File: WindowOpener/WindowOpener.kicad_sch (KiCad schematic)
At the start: 32 parts, among them J1 Conn_ST_STDC14, J2 UEXT_Host, SW1 SW_Push, SW2 SW_SPDT_XKB, U1 STM32L152RCTxA, Y1 8MHz, Y2 32.768kHz

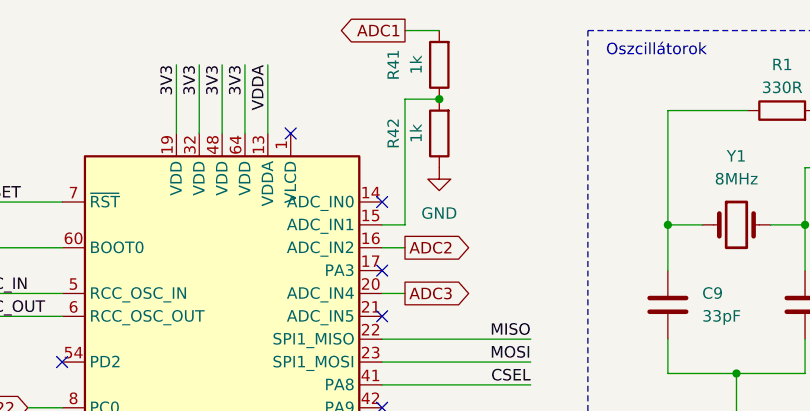
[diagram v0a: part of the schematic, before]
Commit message: v0.5
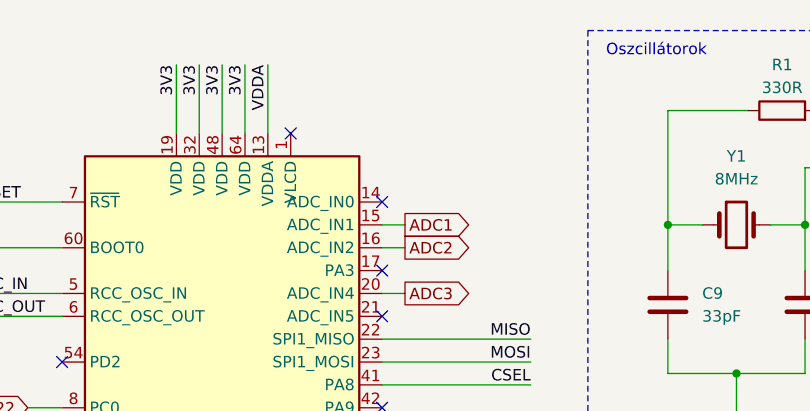
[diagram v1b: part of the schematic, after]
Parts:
- removed R41, R42: 1k, Resistor_SMD:R_2010_5025Metric_Pad1.40x2.65mm_HandSolder, symbol Device:R
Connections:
- net ADC1: now also U1.15 (PA1)

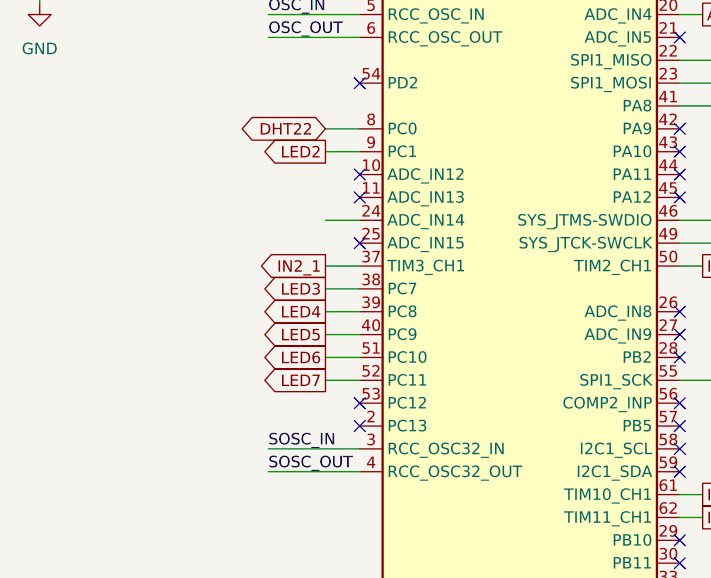
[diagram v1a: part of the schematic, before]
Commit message: v0.6
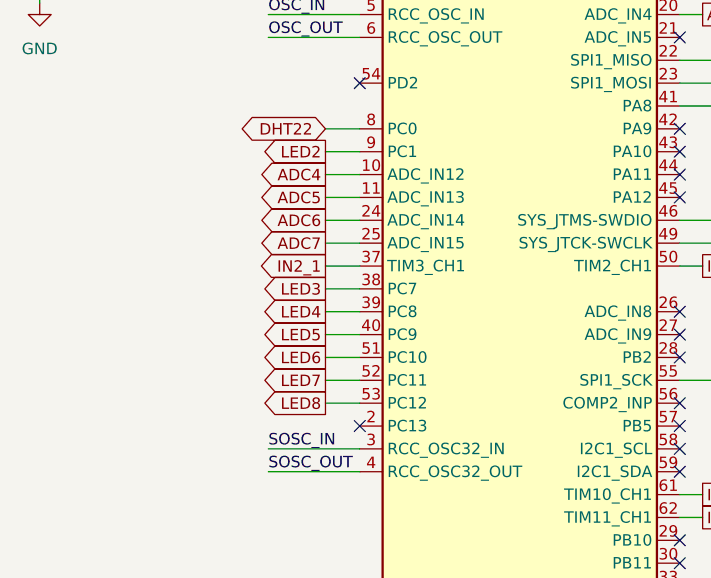
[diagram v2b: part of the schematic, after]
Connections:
- net ADC4: now reaches U1.10 (PC2)
- net ADC5: now reaches U1.11 (PC3)
- net ADC6: now reaches U1.24 (PC4)
- net ADC7: now reaches U1.25 (PC5)
- net LED8: now reaches U1.53 (PC12)
- no-connect marks 27 -> 23
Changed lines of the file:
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@@
-	)
-	(no_connect
-		(at 76.2 86.36)
 	)
 	(no_connect
@@
 	)
 	(no_connect
-		(at 76.2 60.96)
-	)
-	(no_connect
 		(at 111.76 86.36)
 	)
@@
 	)
 	(no_connect
-		(at 76.2 68.58)
-	)
-	(no_connect
 		(at 111.76 55.88)
 	)
@@
 		(at 111.76 63.5)
 	)
-	(no_connect
-		(at 76.2 63.5)
-	)
 	(wire
 		(pts
@@
 	(wire
 		(pts
+			(xy 72.39 60.96) (xy 76.2 60.96)
+		)
+		(stroke
+			(width 0)
+			(type default)
+		)
+	)
+	(wire
+		(pts
 			(xy 96.52 17.78) (xy 96.52 25.4)
 		)
@@
 	(wire
 		(pts
+			(xy 72.39 66.04) (xy 76.2 66.04)
+		)
+		(stroke
+			(width 0)
+			(type default)
+		)
+	)
+	(wire
+		(pts
 			(xy 182.88 107.95) (xy 185.42 107.95)
 		)
@@
 	(wire
 		(pts
+			(xy 72.39 68.58) (xy 76.2 68.58)
+		)
+		(stroke
+			(width 0)
+			(type default)
+		)
+	)
+	(wire
+		(pts
 			(xy 271.78 120.65) (xy 280.67 120.65)
 		)
@@
 	(wire
 		(pts
+			(xy 72.39 63.5) (xy 76.2 63.5)
+		)
+		(stroke
+			(width 0)
+			(type default)
+		)
+	)
+	(wire
+		(pts
 			(xy 72.39 58.42) (xy 76.2 58.42)
 		)
@@
 	(wire
 		(pts
+			(xy 72.39 86.36) (xy 76.2 86.36)
+		)
+		(stroke
+			(width 0)
+			(type default)
+		)
+	)
+	(wire
+		(pts
 			(xy 165.1 118.11) (xy 167.64 118.11)
 		)
@@
 		(pts
 			(xy 250.19 44.45) (xy 250.19 49.53)
-		)
-		(stroke
-			(width 0)
-			(type default)
-		)
-	)
-	(wire
-		(pts
-			(xy 72.39 66.04) (xy 76.2 66.04)
 		)
 		(stroke
@@
 			)
 			(justify left bottom)
+		)
+	)
+	(global_label "LED8"
+		(shape output)
+		(at 72.39 86.36 180)
+		(fields_autoplaced yes)
+		(effects
+			(font
+				(size 1.27 1.27)
+			)
+			(justify right)
+		)
+		(property "Intersheetrefs" "${INTERSHEET_REFS}"
+			(at 64.7482 86.36 0)
+			(effects
+				(font
+					(size 1.27 1.27)
+				)
+				(justify right)
+				(hide yes)
+			)
+		)
+	)
+	(global_label "ADC5"
+		(shape output)
+		(at 72.39 63.5 180)
+		(fields_autoplaced yes)
+		(effects
+			(font
+				(size 1.27 1.27)
+			)
+			(justify right)
+		)
+		(property "Intersheetrefs" "${INTERSHEET_REFS}"
+			(at 64.5667 63.5 0)
+			(effects
+				(font
+					(size 1.27 1.27)
+				)
+				(justify right)
+				(hide yes)
+			)
 		)
 	)
@@
 		)
 	)
+	(global_label "ADC4"
+		(shape output)
+		(at 72.39 60.96 180)
+		(fields_autoplaced yes)
+		(effects
+			(font
+				(size 1.27 1.27)
+			)
+			(justify right)
+		)
+		(property "Intersheetrefs" "${INTERSHEET_REFS}"
+			(at 64.5667 60.96 0)
+			(effects
+				(font
+					(size 1.27 1.27)
+				)
+				(justify right)
+				(hide yes)
+			)
+		)
+	)
 	(global_label "ADC2"
 		(shape output)
@@
 		)
 	)
+	(global_label "ADC7"
+		(shape output)
+		(at 72.39 68.58 180)
+		(fields_autoplaced yes)
+		(effects
+			(font
+				(size 1.27 1.27)
+			)
+			(justify right)
+		)
+		(property "Intersheetrefs" "${INTERSHEET_REFS}"
+			(at 64.5667 68.58 0)
+			(effects
+				(font
+					(size 1.27 1.27)
+				)
+				(justify right)
+				(hide yes)
+			)
+		)
+	)
 	(global_label "LED7"
 		(shape output)
@@
 			(effects
 				(font
+					(size 1.27 1.27)
+				)
+				(justify right)
+				(hide yes)
+			)
+		)
+	)
+	(global_label "ADC6"
+		(shape output)
+		(at 72.39 66.04 180)
+		(fields_autoplaced yes)
+		(effects
+			(font
+				(size 1.27 1.27)
+			)
+			(justify right)
+		)
+		(property "Intersheetrefs" "${INTERSHEET_REFS}"
+			(at 64.5667 66.04 0)
+			(effects
+				(font

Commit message: v0.7
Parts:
- Y2: footprint Crystal:Crystal_C26-LF_D2.1mm_L6.5mm_Horizontal -> Crystal:Crystal_C26-LF_D2.1mm_L6.5mm_Vertical
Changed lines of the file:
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@@
 			)
 		)
-		(property "Footprint" "Crystal:Crystal_C26-LF_D2.1mm_L6.5mm_Horizontal"
+		(property "Footprint" "Crystal:Crystal_C26-LF_D2.1mm_L6.5mm_Vertical"
 			(at 182.88 35.56 0)
 			(effects

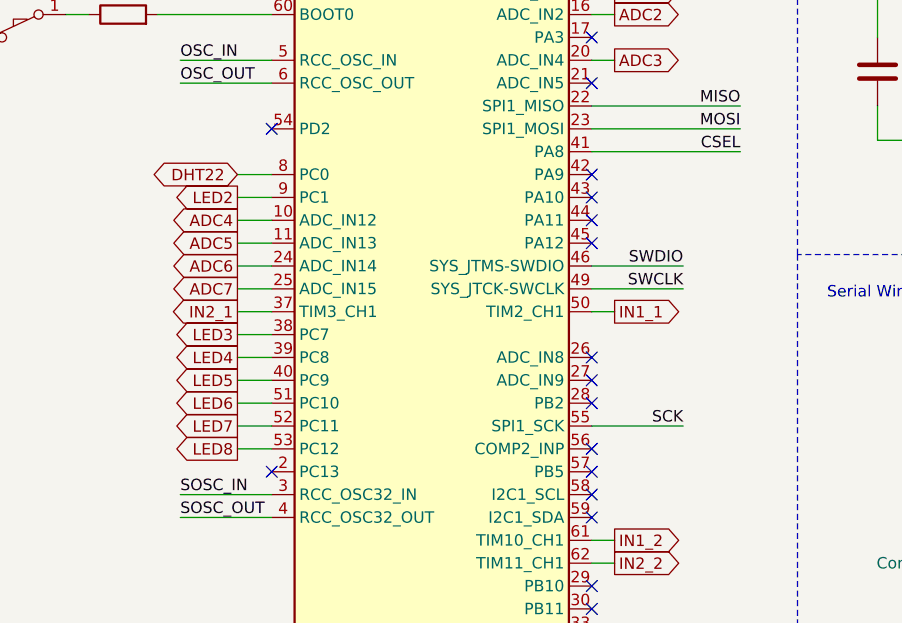
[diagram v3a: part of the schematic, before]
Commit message: v1.0
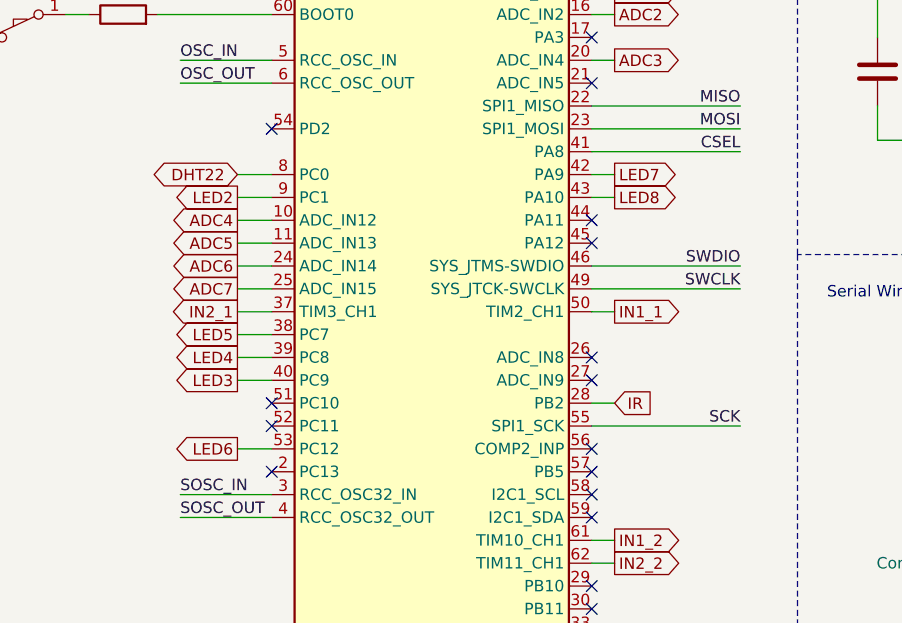
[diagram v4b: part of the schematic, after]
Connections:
- net LED3: now also U1.40 (PC9); no longer U1.38 (PC7)
- net LED5: now also U1.38 (PC7); no longer U1.40 (PC9)
- net LED6: now also U1.53 (PC12); no longer U1.51 (PC10)
- net LED7: now also U1.42 (PA9); no longer U1.52 (PC11)
- net LED8: now also U1.43 (PA10); no longer U1.53 (PC12)
- net IR: now reaches U1.28 (PB2)
- no-connect marks 23 -> 22
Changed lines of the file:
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@@
-	)
-	(no_connect
-		(at 111.76 58.42)
 	)
 	(no_connect
@@
 	)
 	(no_connect
+		(at 76.2 83.82)
+	)
+	(no_connect
 		(at 111.76 109.22)
 	)
@@
 	)
 	(no_connect
-		(at 111.76 55.88)
-	)
-	(no_connect
 		(at 111.76 111.76)
 	)
@@
 	)
 	(no_connect
+		(at 76.2 81.28)
+	)
+	(no_connect
 		(at 111.76 33.02)
 	)
@@
 	)
 	(no_connect
-		(at 111.76 81.28)
-	)
-	(no_connect
 		(at 111.76 106.68)
 	)
@@
 	(wire
 		(pts
-			(xy 111.76 83.82) (xy 121.92 83.82)
+			(xy 111.76 83.82) (xy 128.27 83.82)
 		)
 		(stroke
@@
 	(wire
 		(pts
-			(xy 111.76 68.58) (xy 121.92 68.58)
+			(xy 111.76 68.58) (xy 128.27 68.58)
 		)
 		(stroke
@@
 	(wire
 		(pts
-			(xy 111.76 66.04) (xy 121.92 66.04)
+			(xy 111.76 66.04) (xy 128.27 66.04)
 		)
 		(stroke
@@
 	(wire
 		(pts
+			(xy 111.76 55.88) (xy 114.3 55.88)
+		)
+		(stroke
+			(width 0)
+			(type default)
+		)
+	)
+	(wire
+		(pts
 			(xy 182.88 107.95) (xy 185.42 107.95)
 		)
@@
 	(wire
 		(pts
-			(xy 72.39 81.28) (xy 76.2 81.28)
-		)
-		(stroke
-			(width 0)
-			(type default)
-		)
-	)
-	(wire
-		(pts
 			(xy 175.26 35.56) (xy 175.26 22.86)
 		)
@@
 	(wire
 		(pts
-			(xy 72.39 83.82) (xy 76.2 83.82)
-		)
-		(stroke
-			(width 0)
-			(type default)
-		)
-	)
-	(wire
-		(pts
 			(xy 111.76 96.52) (xy 114.3 96.52)
 		)
@@
 		)
 	)
+	(wire
+		(pts
+			(xy 111.76 58.42) (xy 114.3 58.42)
+		)
+		(stroke
+			(width 0)
+			(type default)
+		)
+	)
 	(polyline
 		(pts
@@
 		(pts
 			(xy 43.18 40.64) (xy 40.64 40.64)
+		)
+		(stroke
+			(width 0)
+			(type default)
+		)
+	)
+	(wire
+		(pts
+			(xy 111.76 81.28) (xy 114.3 81.28)
 		)
 		(stroke
@@
 	)
 	(label "SCK"
-		(at 121.92 83.82 180)
+		(at 128.27 83.82 180)
 		(effects
 			(font
@@
 	)
 	(label "SWCLK"
-		(at 121.92 68.58 180)
+		(at 128.27 68.58 180)
 		(effects
 			(font
@@
 	)
 	(label "SWDIO"
-		(at 121.92 66.04 180)
+		(at 128.27 66.04 180)
 		(effects
 			(font
@@
 	)
 	(global_label "LED8"
+		(shape output)
+		(at 114.3 58.42 0)
+		(fields_autoplaced yes)
+		(effects
+			(font
+				(size 1.27 1.27)
+			)
+			(justify left)
+		)
+		(property "Intersheetrefs" "${INTERSHEET_REFS}"
+			(at 121.9418 58.42 0)
+			(effects
+				(font
+					(size 1.27 1.27)
+				)
+				(justify left)
+				(hide yes)
+			)
+		)
+	)
+	(global_label "LED6"
 		(shape output)
 		(at 72.39 86.36 180)
@@
 		)
 	)
-	(global_label "LED6"
-		(shape output)
-		(at 72.39 81.28 180)
+	(global_label "IR"
+		(shape input)
+		(at 114.3 81.28 0)
 		(fields_autoplaced yes)
 		(effects
@@
 				(size 1.27 1.27)
 			)
-			(justify right)
+			(justify left)
 		)
 		(property "Intersheetrefs" "${INTERSHEET_REFS}"
-			(at 64.7482 81.28 0)
+			(at 119.16 81.28 0)
 			(effects
 				(font
 					(size 1.27 1.27)
 				)
-				(justify right)
+				(justify left)
 				(hide yes)
 			)
 		)
 	)
-	(global_label "LED5"
+	(global_label "LED3"
 		(shape output)
 		(at 72.39 78.74 180)
@@
 		)
 	)
-	(global_label "LED7"
-		(shape output)
-		(at 72.39 83.82 180)
-		(fields_autoplaced yes)
-		(effects
-			(font
-				(size 1.27 1.27)
-			)
-			(justify right)
-		)
-		(property "Intersheetrefs" "${INTERSHEET_REFS}"
-			(at 64.7482 83.82 0)
-			(effects
-				(font
-					(size 1.27 1.27)
-				)
-				(justify right)
-				(hide yes)
-			)
-		)
-	)
 	(global_label "ADC3"
 		(shape output)
@@
 		)
 	)
+	(global_label "LED7"
+		(shape output)
+		(at 114.3 55.88 0)
+		(fields_autoplaced yes)
+		(effects
+			(font
+				(size 1.27 1.27)
+			)
+			(justify left)
+		)
+		(property "Intersheetrefs" "${INTERSHEET_REFS}"
+			(at 121.9418 55.88 0)
+			(effects
+				(font
+					(size 1.27 1.27)
+				)
+				(justify left)
+				(hide yes)
+			)
+		)
+	)
 	(global_label "LED2"
 		(shape output)
@@
 		)
 	)
-	(global_label "LED3"
+	(global_label "LED5"
 		(shape output)
 		(at 72.39 73.66 180)
